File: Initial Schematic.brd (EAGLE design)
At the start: 100 x 58.4 mm, 10 parts, among them J1 CONNECTOR, U1 CAN_TRANSCAN_TRANS, U2 XC6210B332MR-G

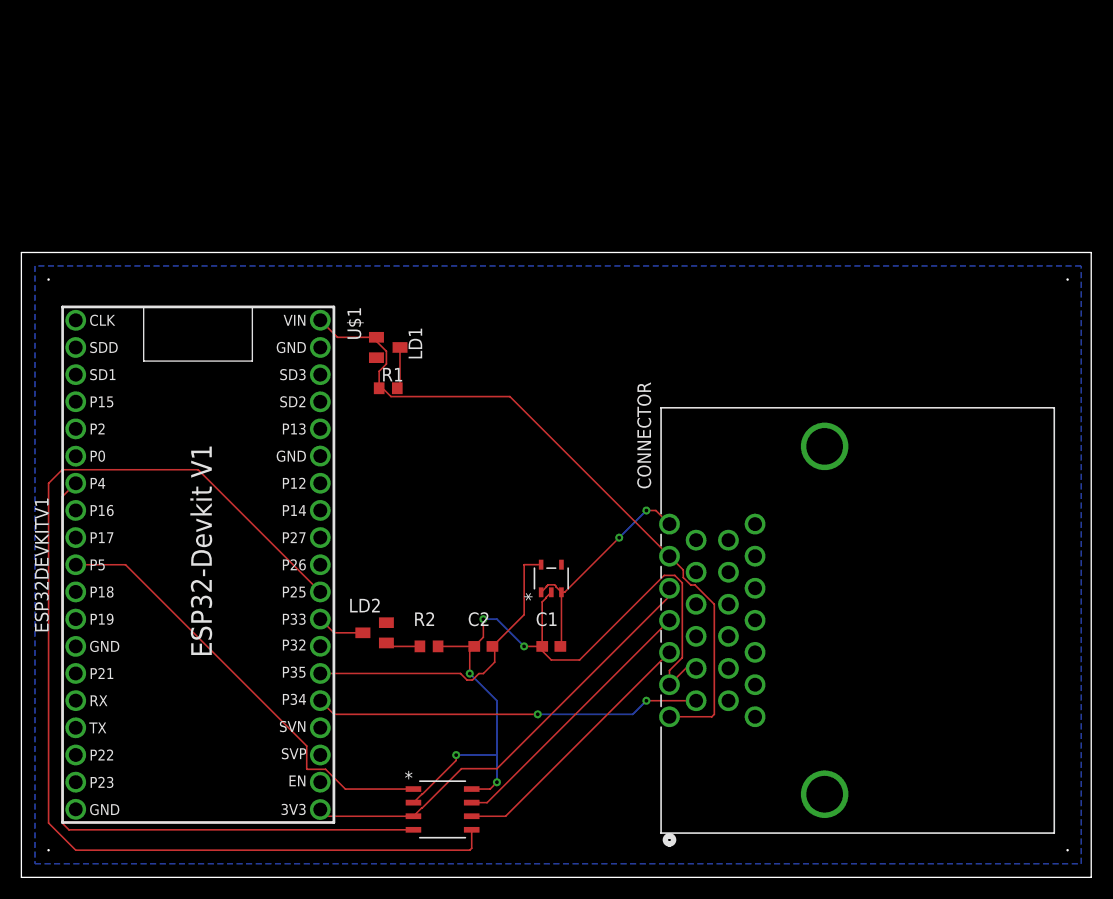
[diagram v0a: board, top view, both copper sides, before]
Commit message: Revised layout
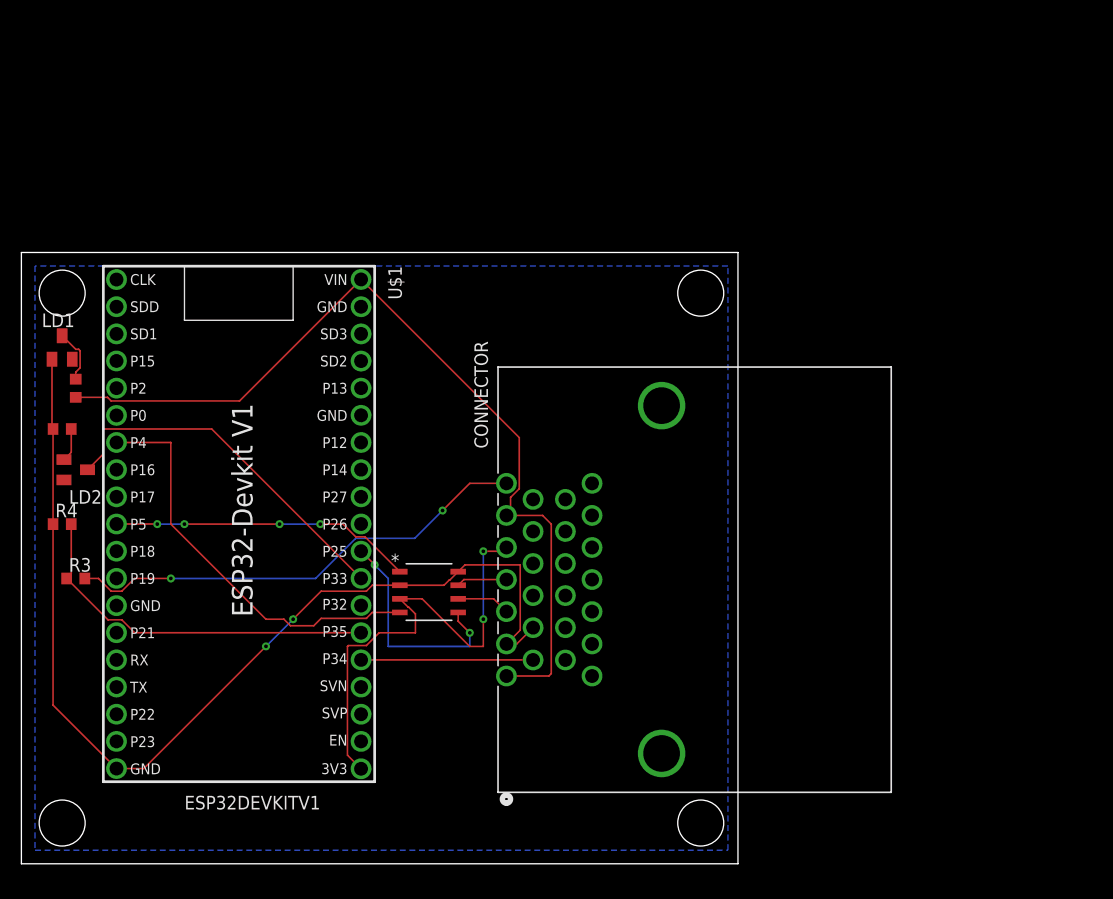
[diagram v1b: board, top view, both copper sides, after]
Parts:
- removed C1, C2: 1.0µF, NFR23:C0603
- removed U2: XC6210B332MR-G, CX6210B332MR-G:SOT-25_TOR
- added R3: 1k, NFR23:R0603
- added R4: 2k, NFR23:R0603
- moved R2 39.9 mm to (3.81, 41.9), turned to 0 degrees
- moved LD2 31.8 mm to (5.08, 38.1), turned to 270 degrees
- moved LD1 30.5 mm to (3.81, 49.5), turned to 0 degrees
- moved R1 29.2 mm to (5.08, 45.7), turned to 90 degrees
- moved U1 20.4 mm to (38.1, 26.7)
- moved J1 15.7 mm to (53.3, 36.8)
- moved U$1 5.39 mm to (21.6, 33.0)
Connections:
- net 5V: no longer LD1.1
- net BRAKE_3V3: now also R3.1, R4.2; no longer C2.1, U2.5
- net BRAKE_5V: now also R3.2; no longer C1.1, U2.1, U2.3
- net GND: now also LD1.1, R4.1; no longer C1.2, C2.2, U2.2
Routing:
- net CAN_SHDN: track 104.8 -> 21.2 mm, vias 0 -> 2
- net N$4: track 4.51 -> 34.3 mm
- net N$3: track 65.4 -> 38.6 mm
- net BRAKE_5V: track 21.4 -> 44.1 mm
- net GND: track 75.3 -> 97.4 mm, vias 5 -> 2
- net CANH: track 25.5 -> 4.74 mm
- net WHEEL_SPEED: track 36.2 -> 16.1 mm, vias 2 -> 0
- net CANL: track 24.8 -> 5.01 mm
- net 5V: track 66.0 -> 82.8 mm
- net N$1: track 41.5 -> 28.3 mm, vias 0 -> 4
- net BRAKE_3V3: track 29.4 -> 34.9 mm
- net 3V3: track 42.2 -> 43.5 mm, vias 0 -> 2
- net N$2: track 3.91 -> 5.08 mm
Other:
- board size 100 x 58.4 mm -> 67 x 57.1 mm

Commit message: Layout v3
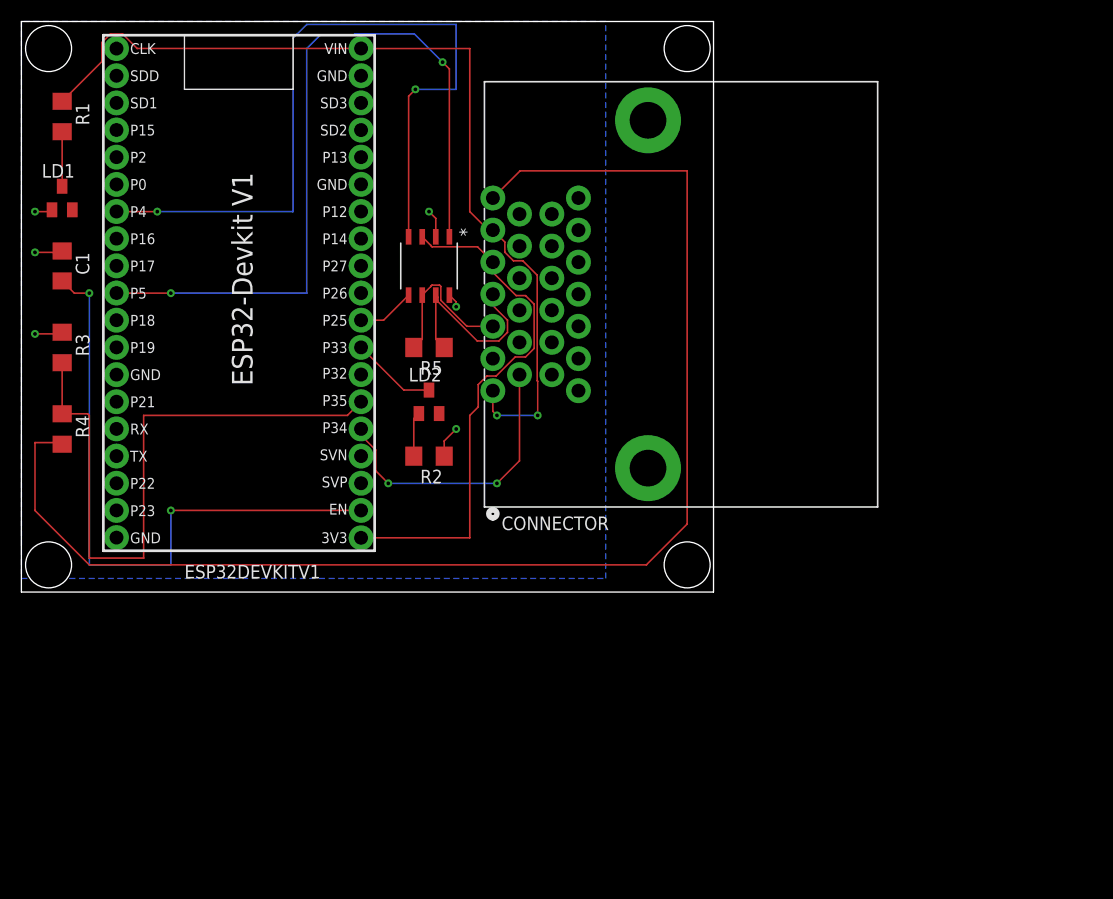
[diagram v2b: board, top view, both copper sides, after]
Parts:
- added C1: 1uF, NFR23:C1206
- added R5: 120, NFR23:R1206
- R1, R2: device NFR23:R0603 -> NFR23:R1206
- R3: value 1k -> 2k; device NFR23:R0603 -> NFR23:R1206
- R4: value 2k -> 1k; device NFR23:R0603 -> NFR23:R1206
- moved R2 34.4 mm to (38.1, 39.4), turned to 180 degrees
- moved LD2 33.6 mm to (38.1, 44.5), turned to 0 degrees
- moved U1 30.5 mm to (38.1, 57.1), turned to 270 degrees
- moved J1 26.7 mm to (52.1, 63.5)
- moved R1 25.4 mm to (3.81, 71.1), turned to 270 degrees
- moved R3 21.6 mm to (3.81, 49.5), turned to 270 degrees
- moved U$1 21.6 mm to (21.6, 54.6)
- moved LD1 14.0 mm to (3.81, 63.5)
- moved R4 8.89 mm to (3.81, 41.9), turned to 270 degrees
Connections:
- new net EN: C1.2, U$1.21
- net BRAKE_3V3: now also R3.2, R4.1; no longer R3.1, R4.2
- net BRAKE_5V: now also R4.2; no longer R3.2
- net CANH: now also R5.1
- net CANL: now also R5.2
- net GND: now also C1.1, R3.1; no longer R4.1
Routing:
- net GND: track 97.4 -> 13.8 mm, vias 2 -> 6
- net BRAKE_5V: track 44.1 -> 125.8 mm, vias 2 -> 0
- net EN: track 0.00 -> 58.9 mm, vias 0 -> 2
- net N$1: track 28.3 -> 71.6 mm, vias 4 -> 2
- net N$3: track 38.6 -> 72.4 mm, vias 0 -> 2
- net N$4: track 34.3 -> 8.00 mm
- net BRAKE_3V3: track 34.9 -> 60.0 mm
- net CAN_SHDN: track 21.2 -> 5.42 mm, vias 2 -> 0
- net CANH: track 4.74 -> 18.4 mm
- net WHEEL_SPEED: track 16.1 -> 27.3 mm, vias 0 -> 2
- net CANL: track 5.01 -> 14.6 mm
- net 3V3: track 43.5 -> 49.2 mm, vias 2 -> 0
- net 5V: track 82.8 -> 86.3 mm, vias 0 -> 2
- net N$5: track 3.14 -> 4.18 mm
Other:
- board size 67 x 57.1 mm -> 64.7 x 53.3 mm
